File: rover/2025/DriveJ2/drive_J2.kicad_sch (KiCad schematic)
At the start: 54 parts, among them J1 USB_C_USB4105-GF-A, J10 Jumper PWR, J2 XT30PW-F, J3 Eth-Horiz, J4 Eth-Horiz, J5 Conn_01x03, J6 Conn_01x02, J8 Conn_01x03, J9 Conn_01x06, SW1 TS09-63-25-WT-160-SMT-TR, SW2 TS09-63-25-WT-160-SMT-TR, SW3 TS09-63-25-WT-160-SMT-TR, SW4 TS09-63-25-WT-160-SMT-TR, U1 TVS-SMDB03CE3, U2 ESP32-S3-WROVER, U3 XT60PM-F, U4 XT60PW-M, U5 LDO-TLV74033PDBVR, U6 SN65HVD232, U7 SN65HVD232, U8 LDO-LM7805MPX/NOPB

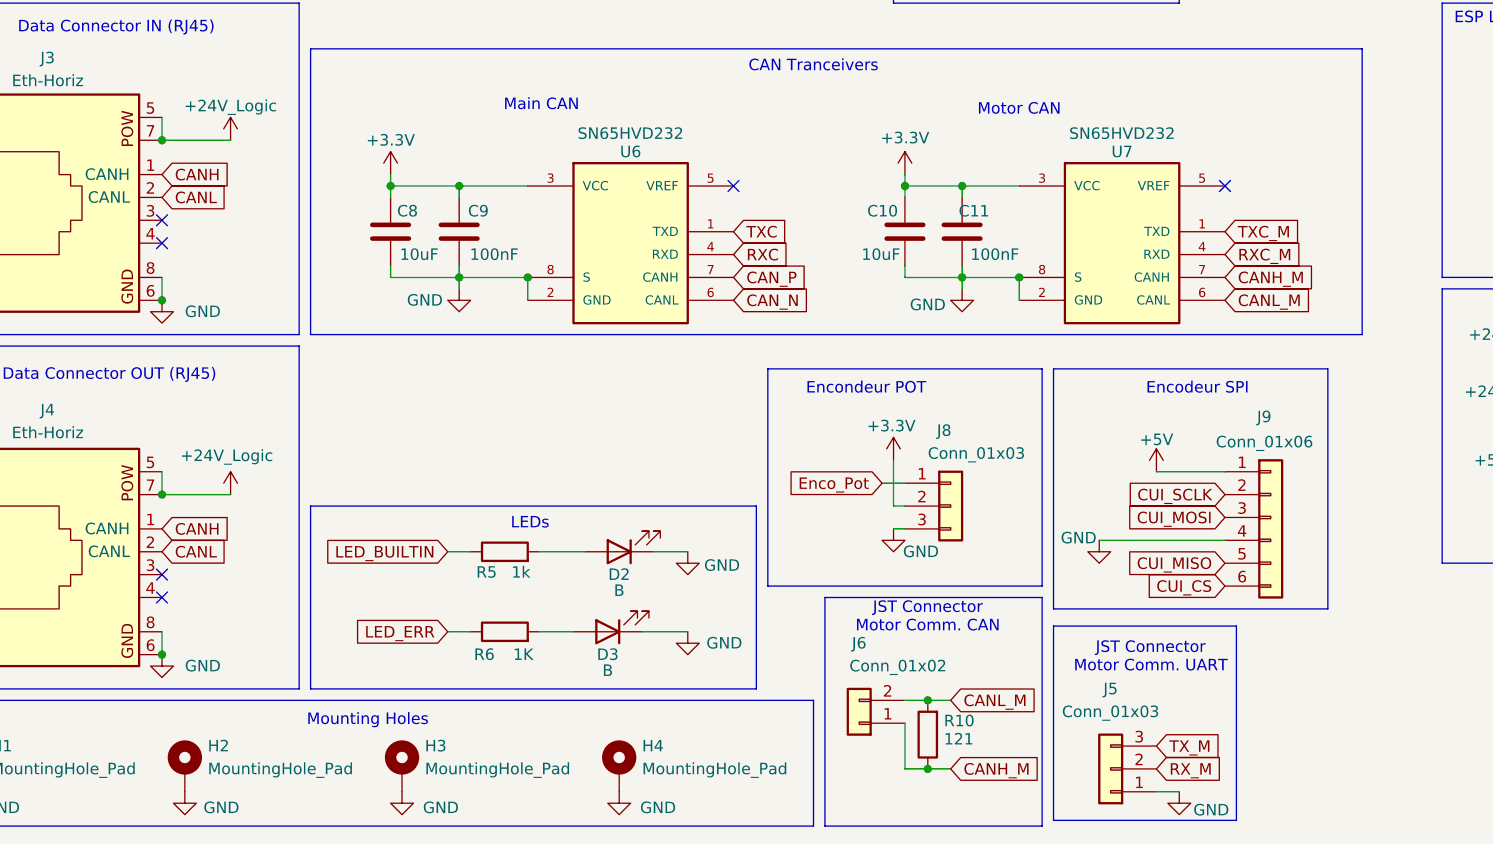
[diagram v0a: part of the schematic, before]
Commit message: Final modifications (DriveJ2)
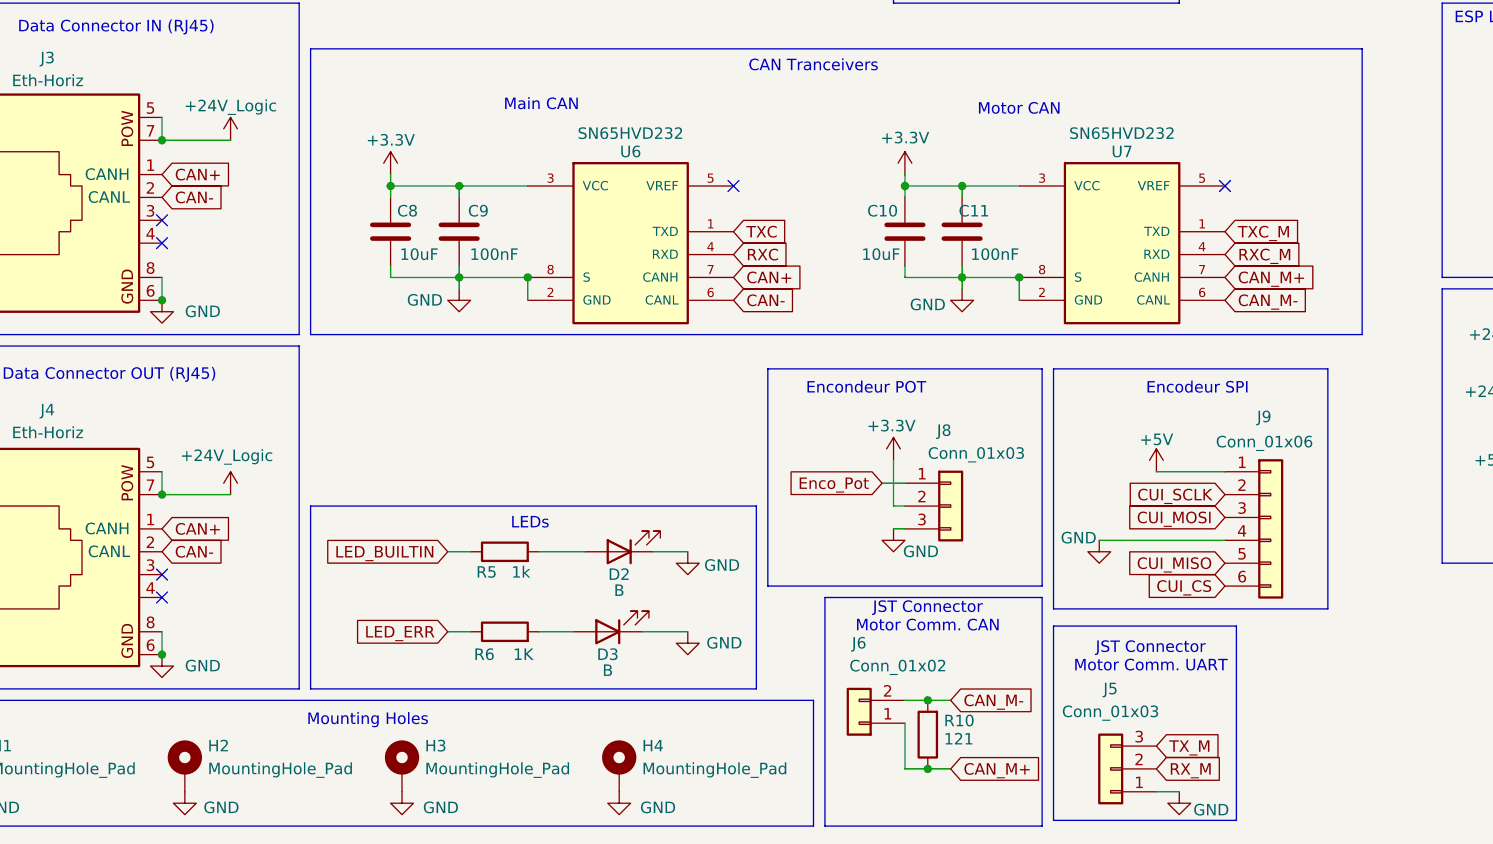
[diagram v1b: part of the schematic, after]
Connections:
- net CAN_N is gone; now on net CAN-: U6.6 (CANL)
- net CAN_P is gone; now on net CAN+: U6.7 (CANH)
- net CANH renamed CAN+
- net CANH_M renamed CAN_M+
- net CANL renamed CAN-
- net CANL_M renamed CAN_M-
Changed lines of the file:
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@@
 		)
 	)
-	(global_label "CANH"
+	(global_label "CAN+"
 		(shape input)
 		(at 39.37 161.29 0)
@@
 		)
 		(property "Intersheetrefs" "${INTERSHEET_REFS}"
-			(at 47.3748 161.29 0)
+			(at 47.6167 161.29 0)
 			(effects
 				(font
@@
 		)
 	)
-	(global_label "CANH_M"
+	(global_label "CAN_M+"
 		(shape input)
 		(at 127 187.96 0)
@@
 		)
 		(property "Intersheetrefs" "${INTERSHEET_REFS}"
-			(at 137.4238 187.96 0)
+			(at 137.6657 187.96 0)
 			(effects
 				(font
@@
 		)
 	)
-	(global_label "CANL_M"
+	(global_label "CAN_M-"
 		(shape input)
 		(at 157.48 135.89 0)
@@
 		)
 		(property "Intersheetrefs" "${INTERSHEET_REFS}"
-			(at 167.6014 135.89 0)
+			(at 168.1457 135.89 0)
 			(effects
 				(font
@@
 		)
 	)
-	(global_label "CANH_M"
+	(global_label "CAN_M+"
 		(shape input)
 		(at 157.48 133.35 0)
@@
 		)
 		(property "Intersheetrefs" "${INTERSHEET_REFS}"
-			(at 167.9038 133.35 0)
-			(effects
-				(font
-					(size 1.27 1.27)
-				)
-				(justify left)
-				(hide yes)
-			)
-		)
-	)
-	(global_label "CANL"
+			(at 168.1457 133.35 0)
+			(effects
+				(font
+					(size 1.27 1.27)
+				)
+				(justify left)
+				(hide yes)
+			)
+		)
+	)
+	(global_label "CAN-"
 		(shape input)
 		(at 39.37 124.46 0)
@@
 		)
 		(property "Intersheetrefs" "${INTERSHEET_REFS}"
-			(at 47.0724 124.46 0)
+			(at 47.6167 124.46 0)
 			(effects
 				(font
@@
 		)
 	)
-	(global_label "CAN_P"
+	(global_label "CAN+"
 		(shape input)
 		(at 102.87 133.35 0)
@@
 		)
 		(property "Intersheetrefs" "${INTERSHEET_REFS}"
-			(at 111.7819 133.35 0)
+			(at 111.1167 133.35 0)
 			(effects
 				(font
@@
 		)
 	)
-	(global_label "CANH"
+	(global_label "CAN+"
 		(shape input)
 		(at 39.37 121.92 0)
@@
 		)
 		(property "Intersheetrefs" "${INTERSHEET_REFS}"
-			(at 47.3748 121.92 0)
+			(at 47.6167 121.92 0)
 			(effects
 				(font
@@
 		)
 	)
-	(global_label "CAN_N"
+	(global_label "CAN-"
 		(shape input)
 		(at 102.87 135.89 0)
@@
 		)
 		(property "Intersheetrefs" "${INTERSHEET_REFS}"
-			(at 111.8424 135.89 0)
+			(at 111.1167 135.89 0)
 			(effects
 				(font
@@
 		)
 	)
-	(global_label "CANL_M"
+	(global_label "CAN_M-"
 		(shape input)
 		(at 127 180.34 0)
@@
 		)
 		(property "Intersheetrefs" "${INTERSHEET_REFS}"
-			(at 137.1214 180.34 0)
+			(at 137.6657 180.34 0)
 			(effects
 				(font
@@
 		)
 	)
-	(global_label "CANL"
+	(global_label "CAN-"
 		(shape input)
 		(at 39.37 163.83 0)
@@
 		)
 		(property "Intersheetrefs" "${INTERSHEET_REFS}"
-			(at 47.0724 163.83 0)
-			(effects
-				(font
+			(at 47.6167 163.83 0)
+			(effects
+				(font
